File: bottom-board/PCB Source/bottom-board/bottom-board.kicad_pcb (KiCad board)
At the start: 4 copper layers, 193 x 93 mm, 307 parts, among them J1 AS0A823-H4SB-7H, P1 USB_B, P10 JACK_TRS_6PINS, P11 JACK_TRS_6PINS, P12 JACK_TRS_6PINS, P13 RJ45, P14 AudioJack3, P2 USB_A, P3 BARREL_JACK, P5 HMI_DATA, P6 AudioJack3, P7 AudioJack3, P8 SERIAL_DEBUG, P9 JACK_TRS_6PINS, Q1 2N7002, Q10 MMBFJ111, Q12 2N7002, Q13 2N7002, Q2 2N7002, Q3 MMBFJ111, Q4 MMBFJ111, Q5 MMBFJ111, Q6 MMBFJ111, Q7 2N7002, Q8 2N7002, Q9 MMBFJ111, U1 TS2596, U10 TPS2001DDBVR, U11 6N137S, U12 ISL83491, U13 AP2120N-3.3, U2 TL750M10CKVURG3, U3 CS4265, U4 AT24CS08-STUM, U5 LM4562, U6 OPA1678, U7 OPA1678, U8 LM4811, U9 LD1117S50TR_SOT223, X1 24.576MHz

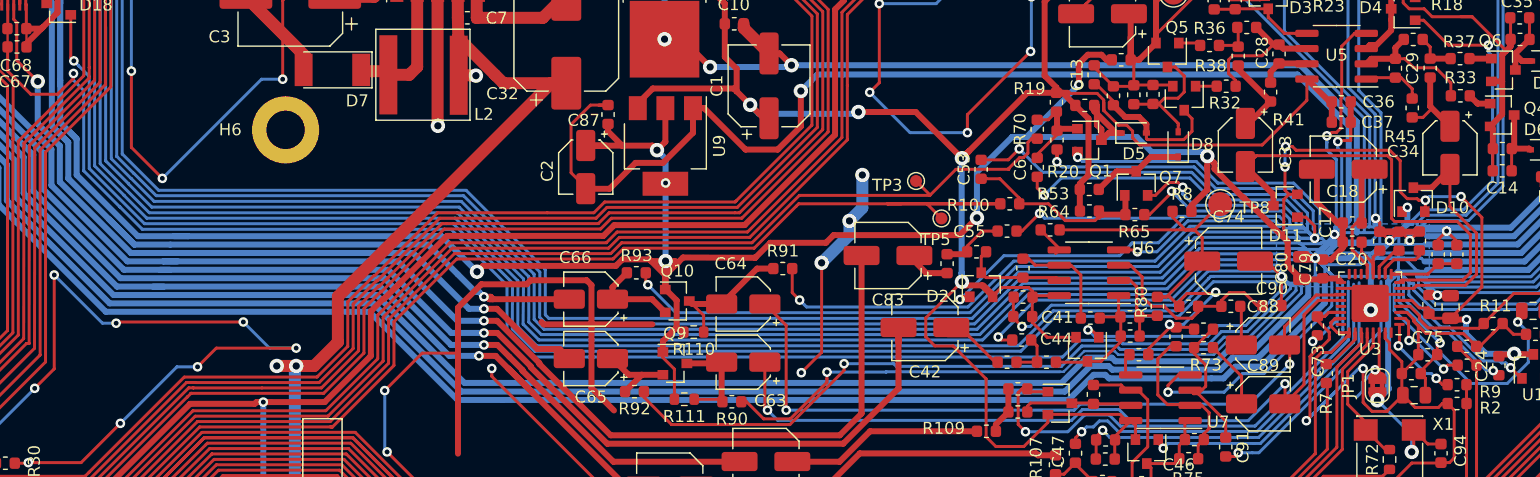
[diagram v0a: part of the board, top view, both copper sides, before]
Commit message: cleanup BOM lines
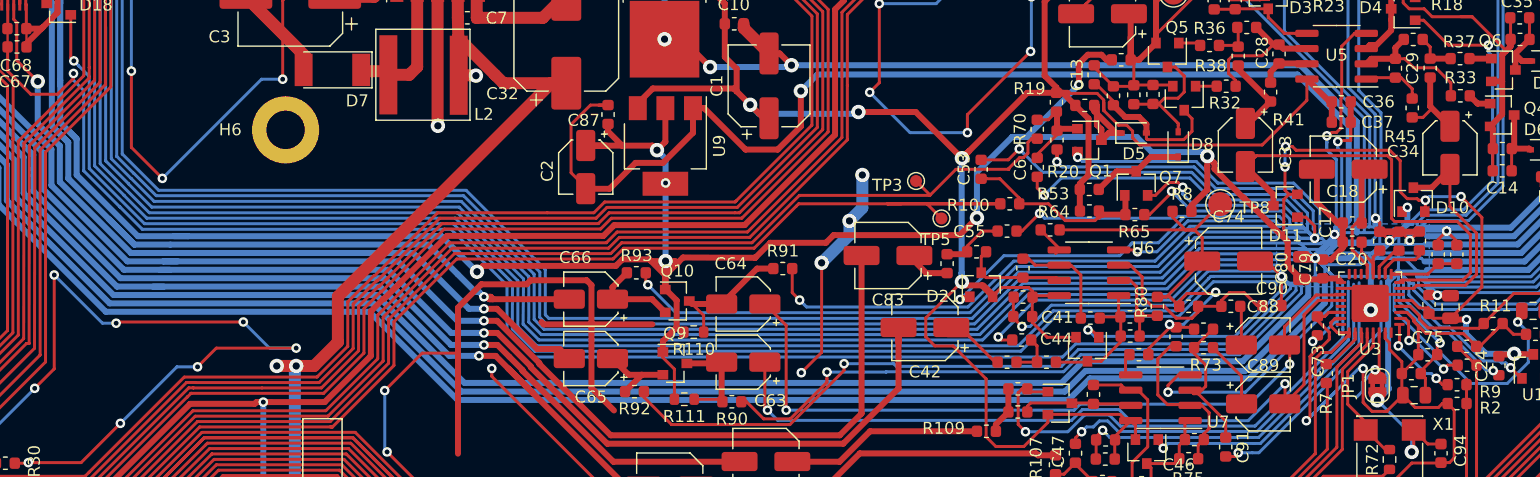
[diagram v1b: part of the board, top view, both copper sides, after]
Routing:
- net GNDA: track 3563.6 -> 3561.3 mm
- net CODEC_I2C_SDA: track 169.7 -> 171.7 mm
